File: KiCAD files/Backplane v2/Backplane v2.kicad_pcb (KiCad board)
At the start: 2 copper layers, 77.5 x 99.1 mm, 10 parts, among them J1 Conn_02x05_Odd_Even, J10 Conn_02x20_Odd_Even, J2 Conn_02x20_Odd_Even, J3 Conn_02x05_Odd_Even, J4 Conn_02x20_Odd_Even, J5 Conn_02x05_Odd_Even, J6 Conn_02x20_Odd_Even, J7 Conn_02x05_Odd_Even, J8 Conn_02x20_Odd_Even, J9 Conn_02x05_Odd_Even

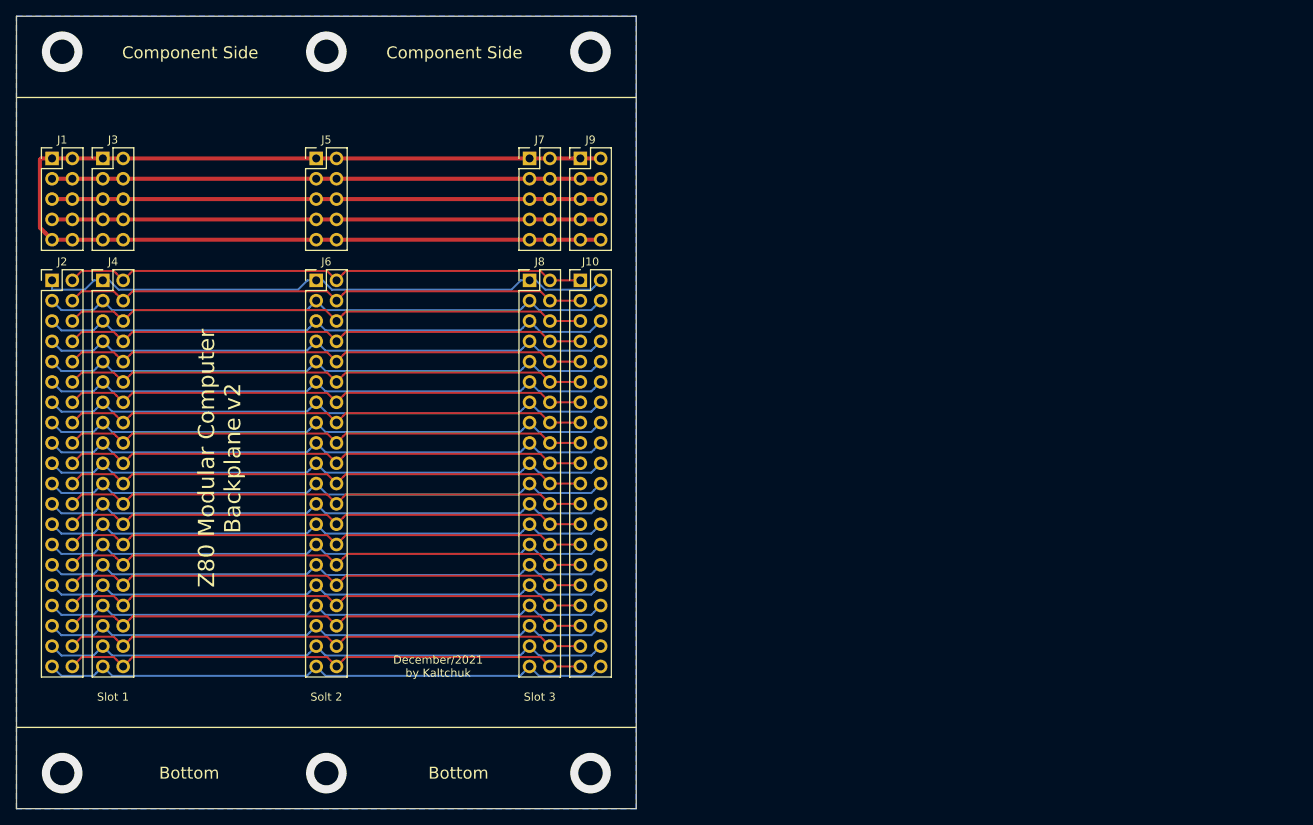
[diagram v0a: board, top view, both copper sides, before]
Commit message: office
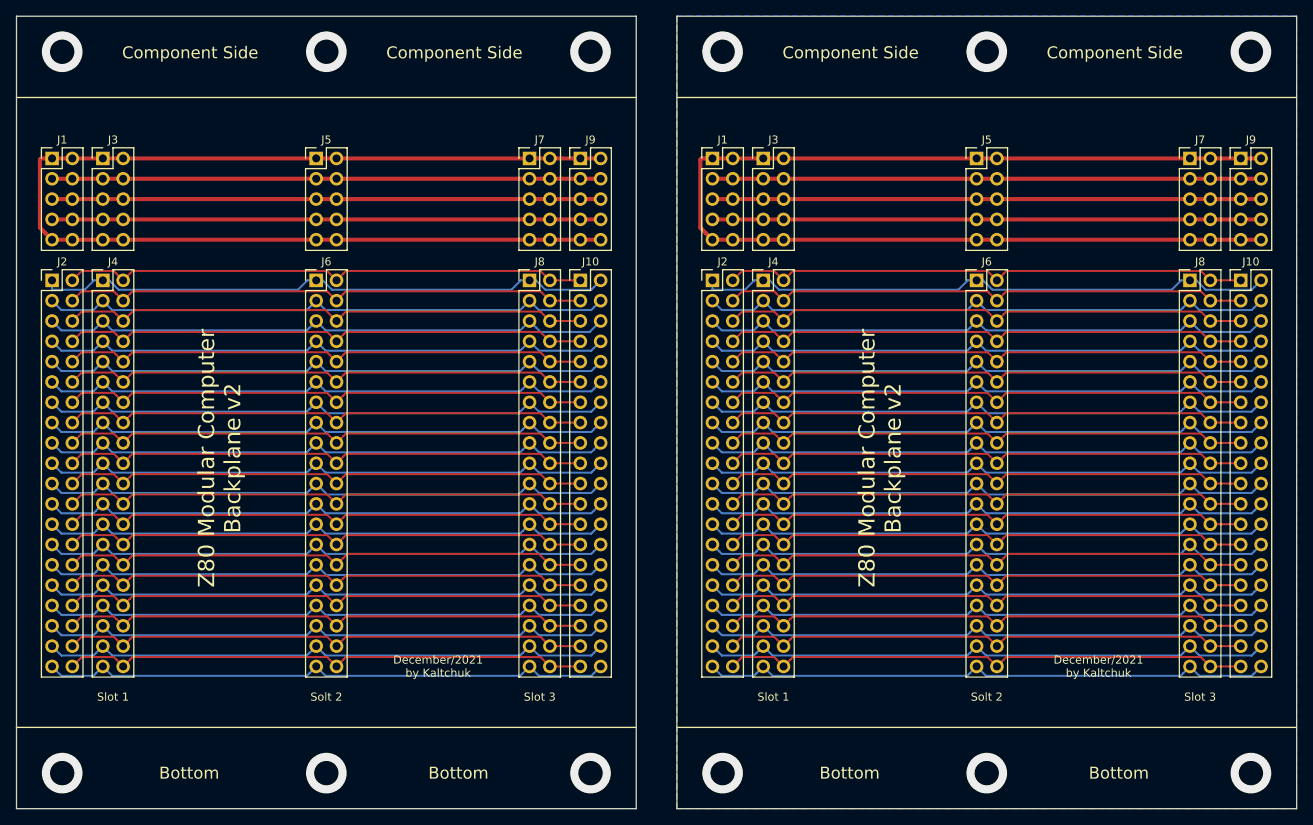
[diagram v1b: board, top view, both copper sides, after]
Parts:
- added J1: Conn_02x05_Odd_Even, Connector_PinHeader_2.54mm:PinHeader_2x05_P2.54mm_Vertical, F.Cu at (170.2, 63.5)
- added J10: Conn_02x20_Odd_Even, Connector_PinHeader_2.54mm:PinHeader_2x20_P2.54mm_Vertical, F.Cu at (236.2, 78.7)
- added J2: Conn_02x20_Odd_Even, Connector_PinHeader_2.54mm:PinHeader_2x20_P2.54mm_Vertical, F.Cu at (170.2, 78.7)
- added J3: Conn_02x05_Odd_Even, Connector_PinHeader_2.54mm:PinHeader_2x05_P2.54mm_Vertical, F.Cu at (176.5, 63.5)
- added J4: Conn_02x20_Odd_Even, Connector_PinHeader_2.54mm:PinHeader_2x20_P2.54mm_Vertical, F.Cu at (176.5, 78.7)
- added J5: Conn_02x05_Odd_Even, Connector_PinHeader_2.54mm:PinHeader_2x05_P2.54mm_Vertical, F.Cu at (203.2, 63.5)
- added J6: Conn_02x20_Odd_Even, Connector_PinHeader_2.54mm:PinHeader_2x20_P2.54mm_Vertical, F.Cu at (203.2, 78.7)
- added J7: Conn_02x05_Odd_Even, Connector_PinHeader_2.54mm:PinHeader_2x05_P2.54mm_Vertical, F.Cu at (229.9, 63.5)
- added J8: Conn_02x20_Odd_Even, Connector_PinHeader_2.54mm:PinHeader_2x20_P2.54mm_Vertical, F.Cu at (229.9, 78.7)
- added J9: Conn_02x05_Odd_Even, Connector_PinHeader_2.54mm:PinHeader_2x05_P2.54mm_Vertical, F.Cu at (236.2, 63.5)
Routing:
- net /gnd: track 149.4 -> 298.7 mm
- net /a00: track 73.1 -> 146.2 mm
- net /a04: track 72.6 -> 145.3 mm
- net /d04: track 72.6 -> 145.3 mm
- net /a12: track 72.6 -> 145.3 mm
- net /busrq: track 72.6 -> 145.1 mm
- net /reset: track 72.5 -> 144.9 mm
- net /a10: track 72.5 -> 144.9 mm
- net /s2: track 72.5 -> 144.9 mm
- net /nmi: track 72.5 -> 144.9 mm
- net /d02: track 72.5 -> 144.9 mm
- net /a14: track 72.5 -> 144.9 mm
- net /wait: track 72.5 -> 144.9 mm
- net /s0: track 72.5 -> 144.9 mm
- net /mreq: track 72.5 -> 144.9 mm
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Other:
- board size 77.5 x 99.1 mm -> 160 x 99.1 mm
